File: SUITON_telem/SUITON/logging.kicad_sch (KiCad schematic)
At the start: 2 parts, among them U6 RFM95W-868S2, U7 W25Q128JVEIQ

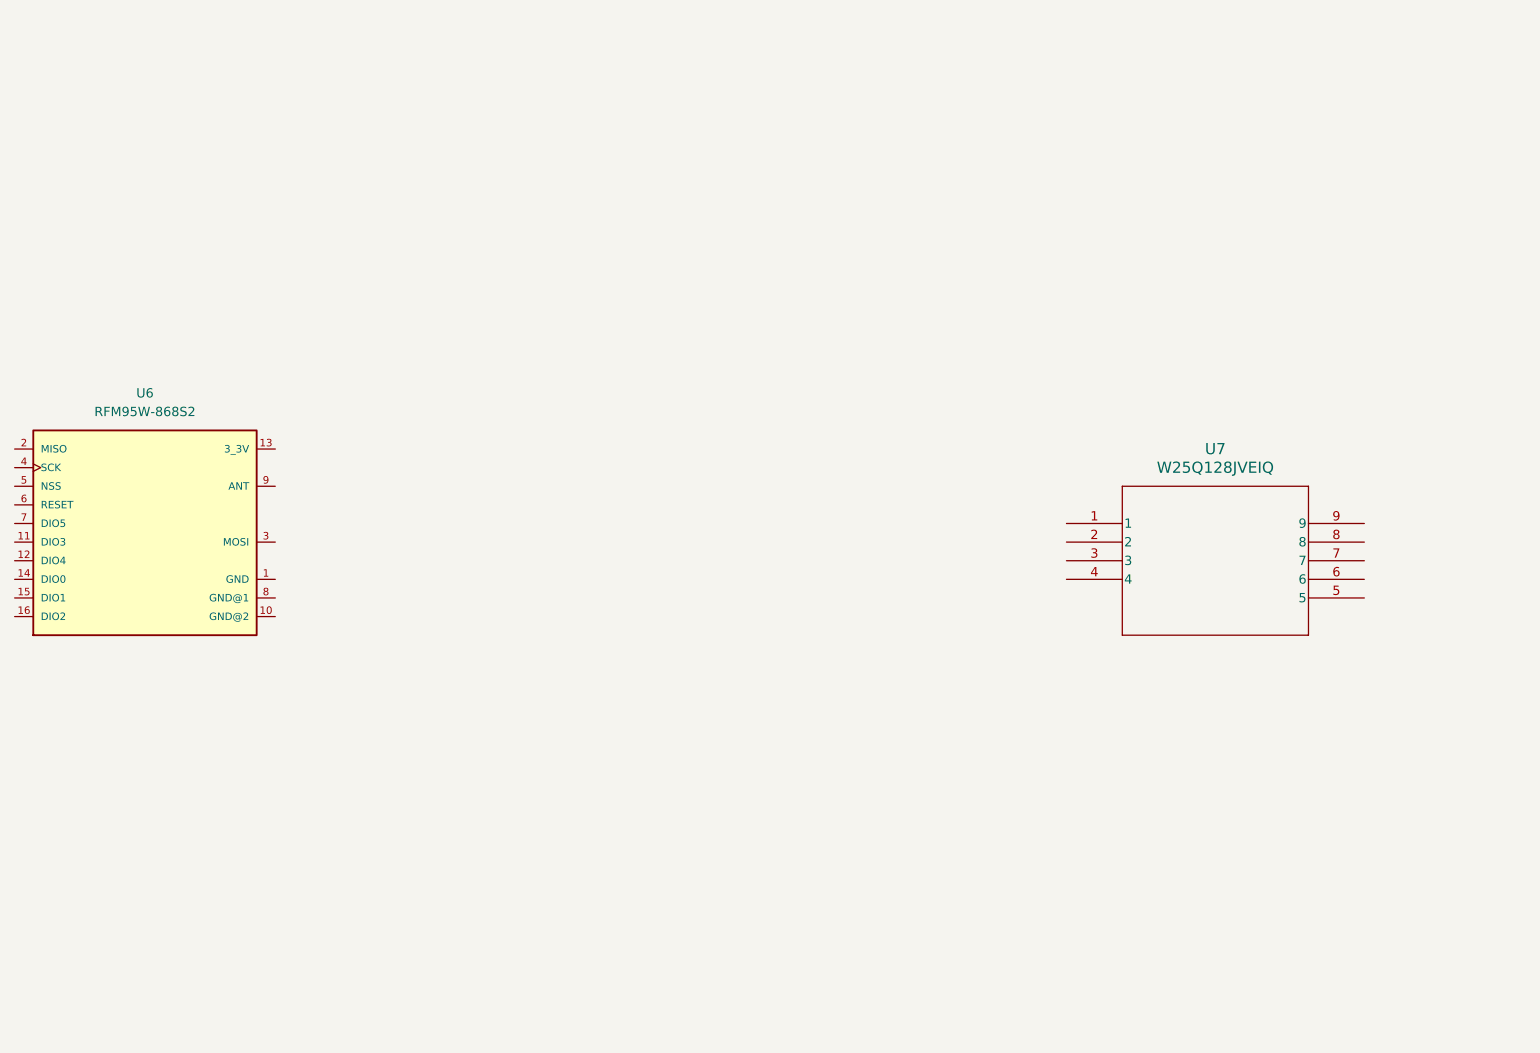
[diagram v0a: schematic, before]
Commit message: power management
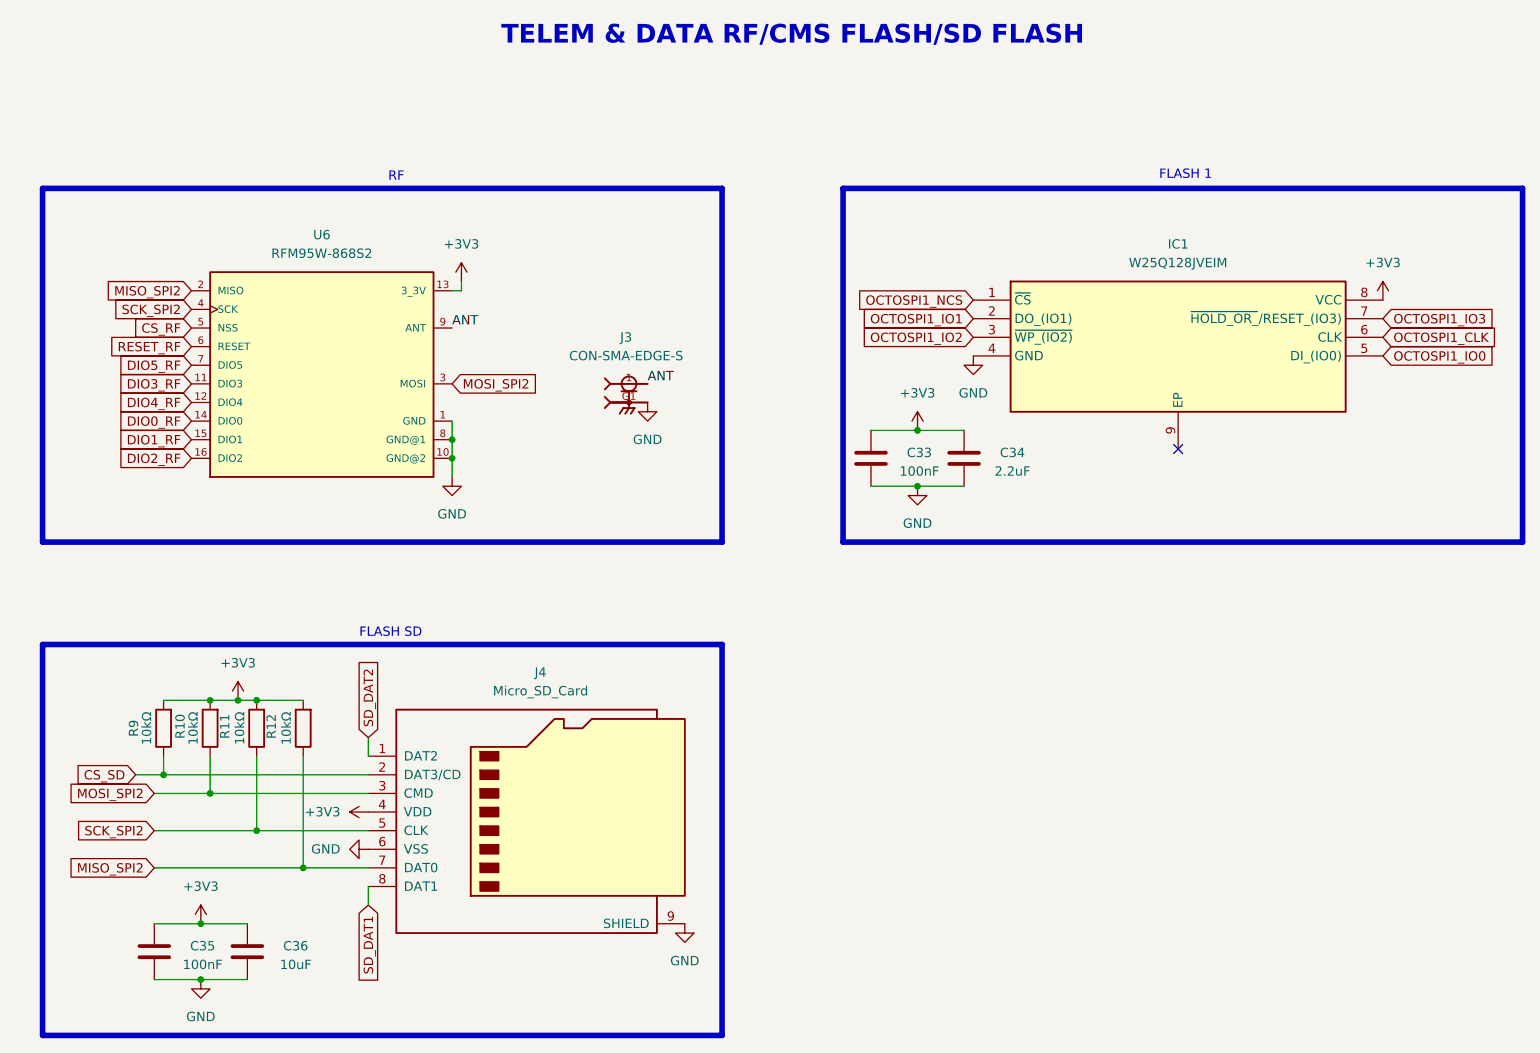
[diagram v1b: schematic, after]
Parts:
- removed U7: W25Q128JVEIQ, WSON_128JVEIQ_WIN, symbol 2026-09-30_11-18-33:W25Q128JVEIQ
- added C33, C35: 100nF, Capacitor_SMD:C_0603_1608Metric, symbol Device:C
- added C34: 2.2uF, Capacitor_SMD:C_0603_1608Metric, symbol Device:C
- added C36: 10uF, Capacitor_SMD:C_0603_1608Metric, symbol Device:C
- added IC1: W25Q128JVEIM, SON127P800X600X80-9N-D, symbol W25Q128JVEIM:W25Q128JVEIM
- added J3: CON-SMA-EDGE-S, CON-SMA-EDGE-S:RFSOLUTIONS_CON-SMA-EDGE-S, symbol CON-SMA-EDGE-S:CON-SMA-EDGE-S
- added J4: Micro_SD_Card, symbol Connector:Micro_SD_Card
- added R10, R11, R12, R9: 10kΩ, symbol Device:R
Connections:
- net GND: now reaches U6.1 (GND)
- net GND: now also U6.10 (GND@2), U6.8 (GND@1), C33.1, C34.1, C35.1, C36.1, IC1.4 (GND), J3.G1, J3.G2, J3.G3, J3.G4, J4.6 (VSS), J4.9 (SHIELD)
- net DIO3_RF: now reaches U6.11 (DIO3)
- net DIO4_RF: now reaches U6.12 (DIO4)
- net +3V3: now reaches U6.13 (3_3V)
- net +3V3: now also C33.2, C34.2, C35.2, C36.2, IC1.8 (VCC), J4.4 (VDD), R10.2, R11.2, R12.2, R9.2
- net DIO0_RF: now reaches U6.14 (DIO0)
- net DIO1_RF: now reaches U6.15 (DIO1)
- net DIO2_RF: now reaches U6.16 (DIO2)
- net MISO_SPI2: now reaches U6.2 (MISO)
- net MISO_SPI2: now also J4.7 (DAT0), R12.1
- net MOSI_SPI2: now reaches U6.3 (MOSI)
- net MOSI_SPI2: now also J4.3 (CMD), R10.1
- net SCK_SPI2: now reaches U6.4 (SCK)
- net SCK_SPI2: now also J4.5 (CLK), R11.1
- net CS_RF: now reaches U6.5 (NSS)
- net RESET_RF: now reaches U6.6 (RESET)
- net DIO5_RF: now reaches U6.7 (DIO5)
- net ANT: now reaches U6.9 (ANT)
- net ANT: now also J3.1
- new net CS_SD: J4.2 (DAT3/CD), R9.1
- new net OCTOSPI1_CLK: IC1.6 (CLK)
- new net OCTOSPI1_IO0: IC1.5 (DI_(IO0))
- new net OCTOSPI1_IO1: IC1.2 (DO_(IO1))
- new net OCTOSPI1_IO2: IC1.3 (~{WP_(IO2)})
- new net OCTOSPI1_IO3: IC1.7 (~{HOLD_OR_}/RESET_(IO3))
- new net OCTOSPI1_NCS: IC1.1 (~{CS})
- new net SD_DAT1: J4.8 (DAT1)
- new net SD_DAT2: J4.1 (DAT2)
- no-connect marks 0 -> 1
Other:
- note added: "FLASH 1"
- note added: "FLASH SD"
- note added: "RF"
- note added: "TELEM & DATA RF/CMS FLASH/SD FLASH"
- company: (none) -> S.T.A.R.
- title: (none) -> SUITON PRO
- moved on the sheet: U6

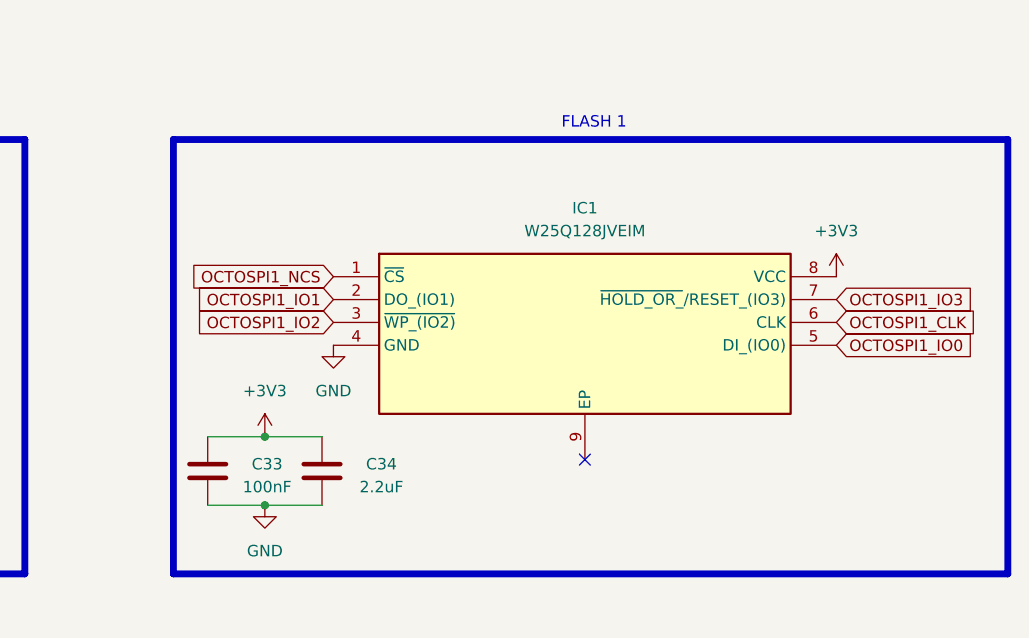
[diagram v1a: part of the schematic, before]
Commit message: SUITON mini
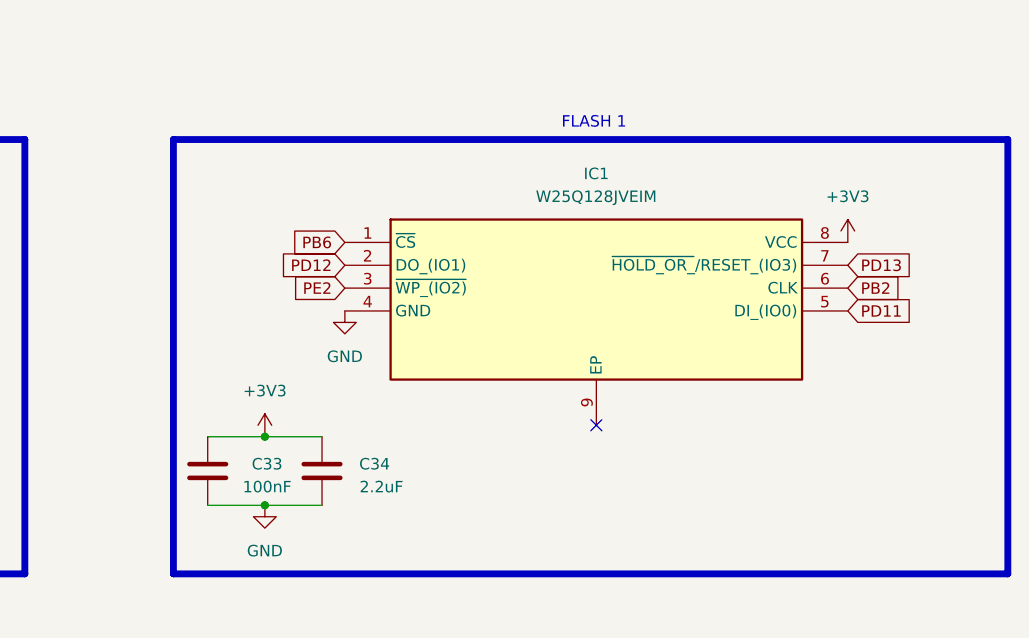
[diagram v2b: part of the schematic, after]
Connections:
- net OCTOSPI1_CLK renamed PB2
- net OCTOSPI1_IO0 renamed PD11
- net OCTOSPI1_IO1 renamed PD12
- net OCTOSPI1_IO2 renamed PE2
- net OCTOSPI1_IO3 renamed PD13
- net OCTOSPI1_NCS renamed PB6
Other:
- moved on the sheet: IC1
